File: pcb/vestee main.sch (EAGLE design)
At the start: 39 parts, among them IC1 LD117AS12TR, IC2 FT232RL, Q1 MMBT2222A, Q3 MMBT4403

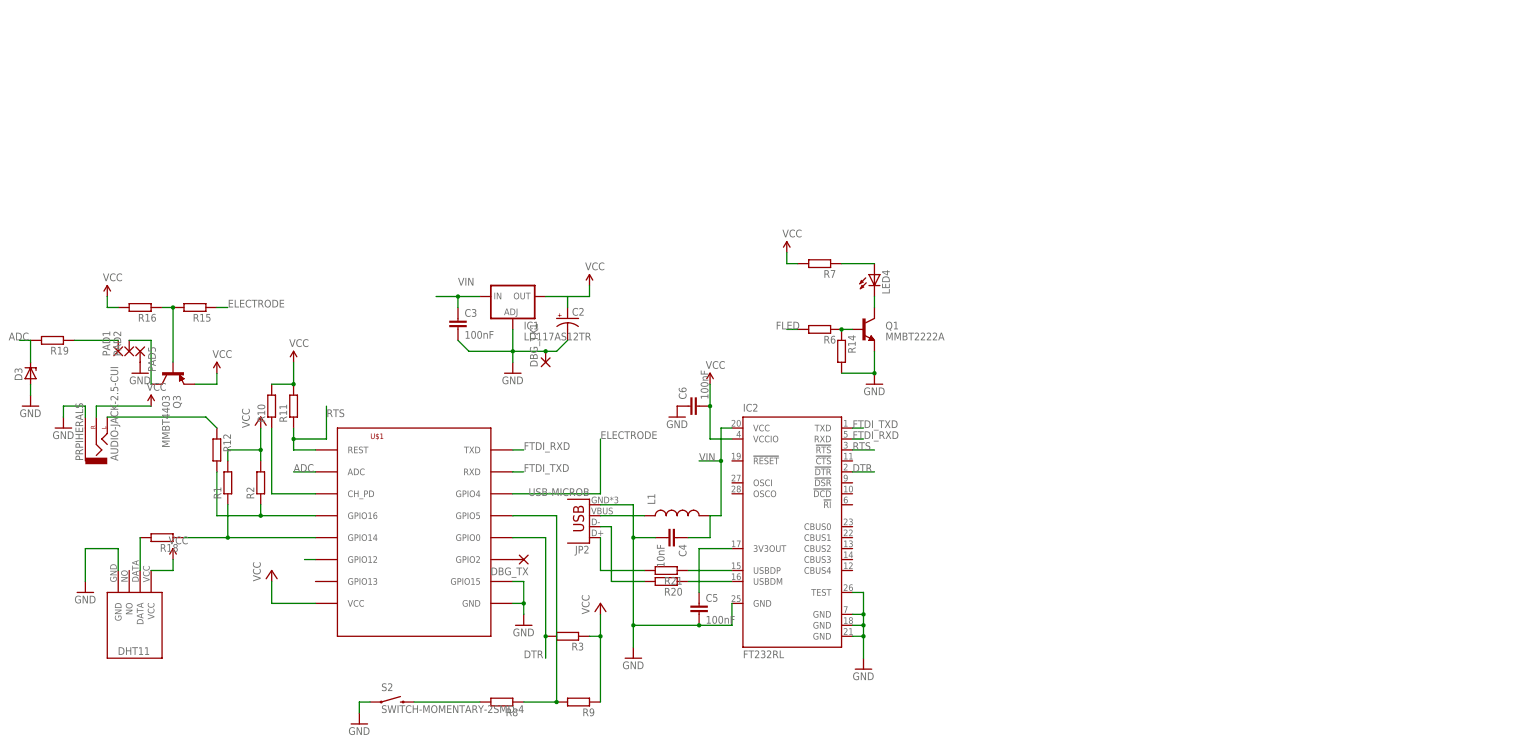
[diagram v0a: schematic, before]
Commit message: pcb rev3
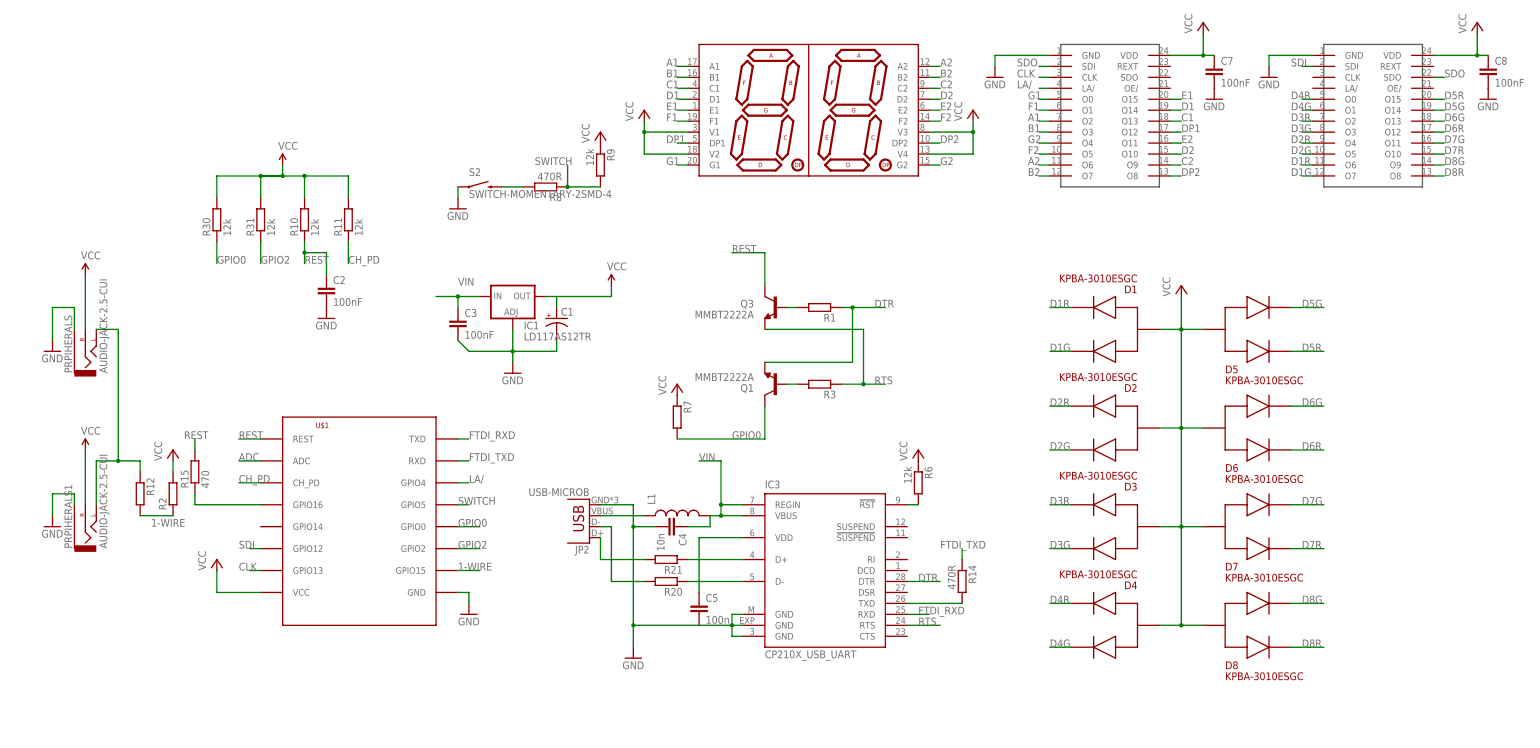
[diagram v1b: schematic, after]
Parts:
- removed C6: 100nF, SparkFun-Capacitors:0.33UF-50V-10%(0805)
- removed DBG_TX, DBG_TX1, PAD1, PAD2, PAD5: (no value), wirepad:SMD2
- removed IC2: FT232RL, ftdichip:FT232RL
- removed LED4: (no value), led:LEDSML0805
- removed R16, R18, R19: (no value), rcl:R-EU_R0805
- added C1: (no value), SparkFun-Passives:CAP_POL3528
- added C7, C8: 100nF, rcl:C-EUC0603
- added D1, D2, D4, D5, D6, D7, D8: KPBA-3010ESGC, SparkFun-LED:APA3010SF4C
- added IC3: CP210X_USB_UART, SparkFun-DigitalIC:CP210X_USB_UART
- added PRPIHERALS1: AUDIO-JACK-2.5-CUI, SparkFun-Connectors:AUDIO-JACK-2.5-CUI
- added R30, R31: 12k, rcl:R-EU_R0603
- added U$3, U$4: SCT2024CSSG, vestee:SCT2024CSSG
- C2: value (none) -> 100nF; device SparkFun-Capacitors:CAP_POLD -> rcl:C-EUC0603
- C3: device SparkFun-Capacitors:0.33UF-50V-10%(0805) -> rcl:C-EUC0603
- C4: value 10nF -> 10n; device SparkFun-Capacitors:0.33UF-50V-10%(0805) -> rcl:C-EUC0603
- C5: value 100nF -> 100n; device SparkFun-Capacitors:0.33UF-50V-10%(0805) -> rcl:C-EUC0603
- D3: value (none) -> KPBA-3010ESGC; device diode:ZENER-DIODESOD80C -> SparkFun-LED:APA3010SF4C
- Q3: value MMBT4403 -> MMBT2222A; device SparkFun-DiscreteSemi:TRANSISTOR_PNPMMBT4403 -> SparkFun-DiscreteSemi:TRANSISTOR_NPNMMBT2222A
- R1, R12, R2, R20, R21, R3, R7: device rcl:R-EU_R0805 -> rcl:R-EU_R0603
- R10, R11, R6, R9: value (none) -> 12k; device rcl:R-EU_R0805 -> rcl:R-EU_R0603
- R14, R8: value (none) -> 470R; device rcl:R-EU_R0805 -> rcl:R-EU_R0603
- R15: value (none) -> 470; device rcl:R-EU_R0805 -> rcl:R-EU_R0603
- U$2: value (none) -> KCDA02-103; device DHT11:DHT11 -> vestee:KCDA02-103
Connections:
- net N$19 renamed SWITCH
- removed net ELECTRODE: R15.1, U$1.GPIO4
- removed net FLED: R6.2, U$1.GPIO12
- removed net N$1: R1.1, R18.1, U$1.GPIO14
- removed net N$10: Q1.B, R14.1, R6.1
- removed net N$16: LED4.C, Q1.C
- removed net N$17: PAD2.P, Q3.C
- removed net N$21: R10.1, U$1.CH_PD
- removed net N$26: PAD1.P, R19.1
- removed net N$27: Q3.B, R15.2, R16.1
- removed net N$4: R12.2, R2.1, U$1.GPIO16
- removed net N$6: R18.2, U$2.DATA
- new net A1: U$2.A1, U$3.O2
- new net A2: U$2.A2, U$3.O6
- new net B1: U$2.B1, U$3.O3
- new net B2: U$2.B2, U$3.O7
- new net C1: U$2.C1, U$3.O13
- new net C2: U$2.C2, U$3.O9
- new net CH_PD: R11.1, U$1.CH_PD
- new net CLK: U$1.GPIO13, U$3.CLK
- new net D1: U$2.D1, U$3.O14
- new net D1G: D1.3, U$4.O7
- new net D1R: D1.2, U$4.O6
- new net D2: U$2.D2, U$3.O10
- new net D2G: D2.3, U$4.O5
- new net D2R: D2.2, U$4.O4
- new net D3G: D3.3, U$4.O3
- new net D3R: D3.2, U$4.O2
- new net D4G: D4.3, U$4.O1
- new net D4R: D4.2, U$4.O0
- new net D5G: D5.3, U$4.O14
- new net D5R: D5.2, U$4.O15
- new net D6G: D6.3, U$4.O13
- new net D6R: D6.2, U$4.O12
- new net D7G: D7.3, U$4.O11
- new net D7R: D7.2, U$4.O10
- new net D8G: D8.3, U$4.O9
- new net D8R: D8.2, U$4.O8
- new net DP1: U$2.DP1, U$3.O12
- new net DP2: U$2.DP2, U$3.O8
- new net E1: U$2.E1, U$3.O15
- new net E2: U$2.E2, U$3.O11
- new net F1: U$2.F1, U$3.O1
- new net F2: U$2.F2, U$3.O5
- new net G1: U$2.G1, U$3.O0
- new net G2: U$2.G2, U$3.O4
- new net GPIO0: Q1.C, R30.1, R7.2, U$1.GPIO0
- new net GPIO16: R15.1, U$1.GPIO16
- new net GPIO2: R31.1, U$1.GPIO2
- new net JACK: PRPIHERALS.LEFT, PRPIHERALS1.LEFT, R12.1
- new net LA/: U$1.GPIO4, U$3.LA/
- new net N$14: IC3.!RST, R6.2
- new net REST: C2.1, Q3.C, R10.1, R15.2, U$1.REST
- new net SDI: U$1.GPIO12, U$4.SDI
- new net SDO: U$3.SDI, U$4.SDO
- new net TXD: IC3.TXD, R14.2
- net 1-WIRE: now also R12.2, R2.1, U$1.GPIO15; no longer PRPIHERALS.LEFT, R12.1
- net ADC: no longer D3.C, R19.2
- net DTR: now also IC3.DTR, Q1.E, R1.1; no longer IC2.!DTR, R3.2, U$1.GPIO0
- net FTDI_RXD: now also IC3.RXD; no longer IC2.RXD
- net FTDI_TXD: now also R14.1; no longer IC2.TXD
- net GND: now also C1.-, C2.2, C7.2, C8.2, IC3.GND, IC3.GND@EXP, IC3.GND@M, PRPIHERALS1.SLEEVE, U$3.GND, U$4.GND; no longer C2.-, C6.1, D3.A, DBG_TX1.P, IC2.GND, IC2.GND@1, IC2.GND@2, IC2.GND@A, IC2.TEST, PAD5.P, Q1.E, R14.2, U$1.GPIO15, U$2.GND
- net N$15: now also Q1.B, R3.2; no longer LED4.A, R7.1
- net N$28: now also IC3.D+; no longer IC2.USBDP
- net N$29: now also IC3.D-; no longer IC2.USBDM
- net N$5: now also Q3.B, R1.2; no longer DBG_TX.P, U$1.GPIO2
- net N$9: now also IC3.VDD; no longer IC2.3V3OUT
- net RTS: now also IC3.RTS, Q3.E, R3.1; no longer IC2.!RTS, R11.1, U$1.REST
- net VCC: now also C1.+, C7.1, C8.1, D1.COM, D2.COM, D3.COM, D4.COM, D5.COM, D6.COM, D7.COM, D8.COM, PRPIHERALS1.RIGHT, R30.2, R31.2, R6.1, R7.1, U$2.V1, U$2.V2, U$2.V3, U$2.V4, U$3.VDD, U$4.VDD; no longer C2.+, C6.2, IC2.VCCIO, Q3.E, R1.2, R16.2, R3.1, R7.2, U$2.VCC
- net VIN: now also IC3.REGIN, IC3.VBUS; no longer IC2.VCC
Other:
- moved on the sheet: C4, PRPIHERALS, Q1, Q3, R1, R10, R11, R12, R14, R15, R2, R21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
